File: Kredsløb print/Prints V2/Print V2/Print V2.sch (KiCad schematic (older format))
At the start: 77 parts, among them J1 Conn_01x01_Male, J10 Conn_01x01_Male, J11 Conn_01x01_Male, J12 Conn_01x01_Male, J13 Conn_01x01_Male, J14 Conn_01x01_Male, J15 Conn_01x01_Male, J16 Conn_01x01_Male, J17 Conn_01x01_Male, J18 Conn_01x01_Male, J19 Conn_01x01_Male, J2 Conn_01x01_Male, J20 Conn_01x01_Male, J21 Conn_01x01_Male, J22 Conn_01x01_Male, J23 Conn_01x01_Male, J24 Conn_01x01_Male, J25 Conn_01x01_Male, J26 Conn_01x01_Male, J27 Conn_01x01_Male, J28 Conn_01x01_Male, J29 Conn_01x01_Male, J3 Conn_01x01_Male, J30 Conn_01x01_Male, J31 Conn_01x01_Male, J32 Conn_01x01_Male, J4 Conn_01x01_Male, J5 Conn_01x01_Male, J6 Conn_01x01_Male, J7 Conn_01x01_Male, J8 Conn_01x01_Male, J9 Conn_01x01_Male, Q1 BC547, Q10 TIP120, Q11 TIP127, Q12 TIP120, Q13 TIP127, Q14 TIP120, Q15 BC547, Q16 BC547, Q17 BC547, Q18 TIP127, Q19 TIP120, Q2 BC547, Q20 BC547, Q21 TIP127, Q22 TIP120, Q23 TIP120, Q24 TIP120, Q25 TIP127, Q26 TIP120, Q27 TIP127, Q28 TIP120, Q3 BC547, Q4 TIP127, Q5 TIP120, Q6 BC547, Q7 TIP127, Q8 TIP120, Q9 TIP120, U1 esp32, U2 LM7805_TO220, U3 4049

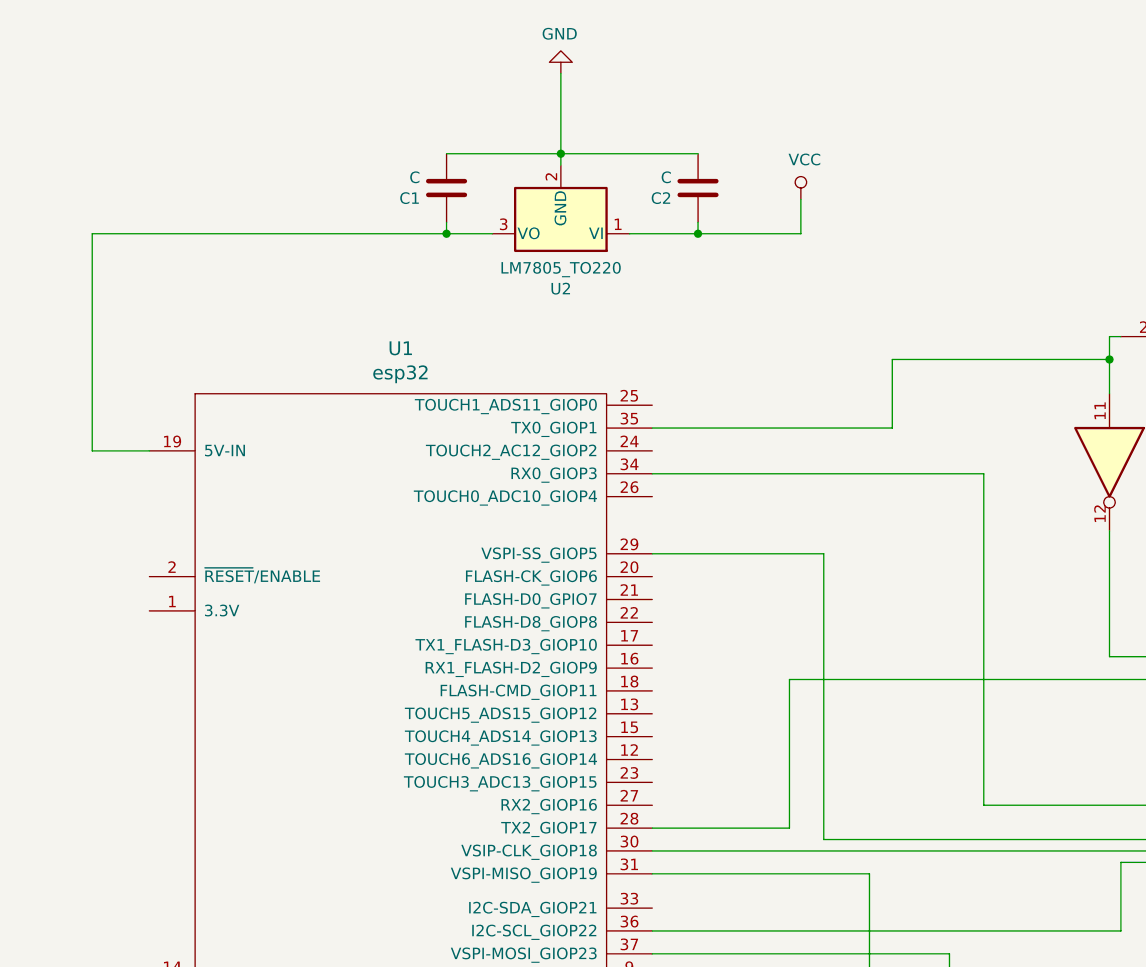
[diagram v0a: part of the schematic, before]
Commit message: kredsløb og ny motor mount
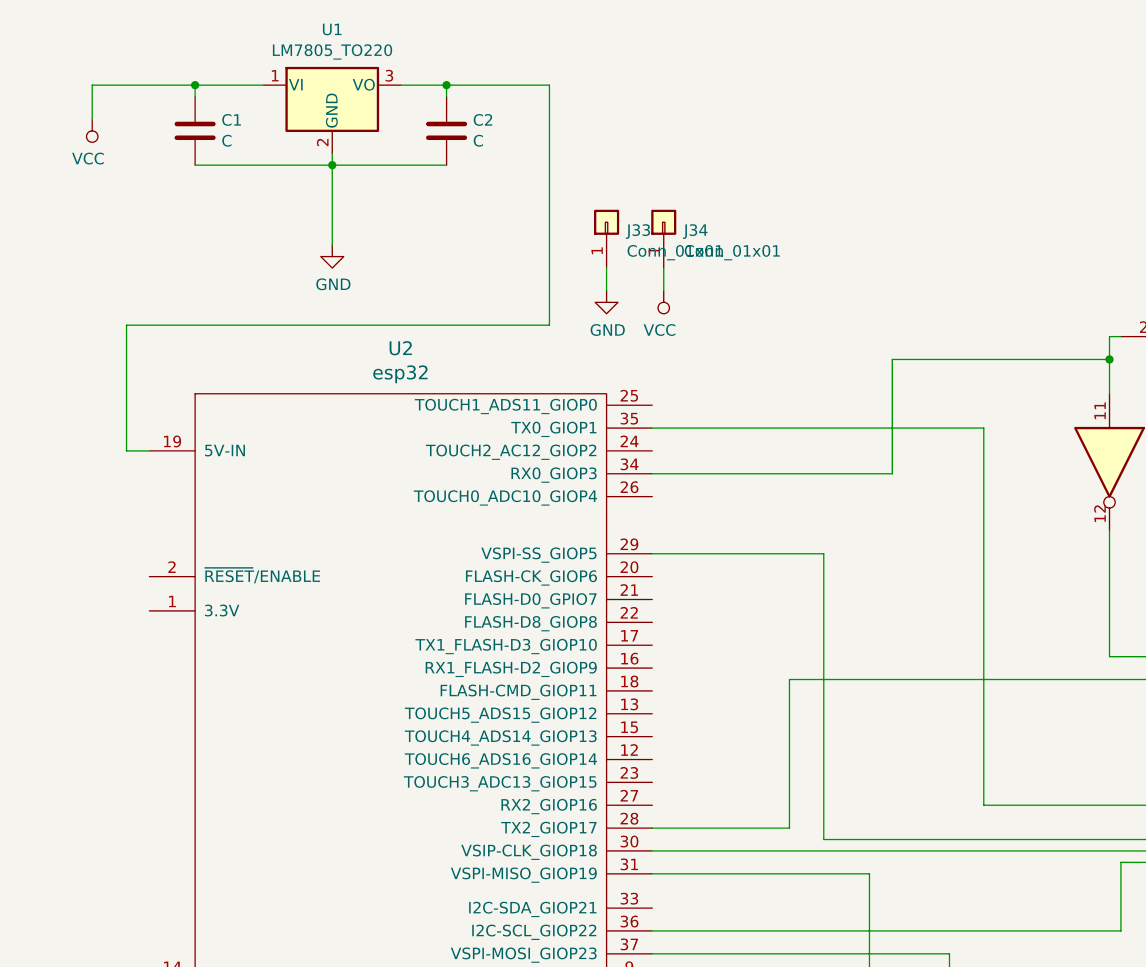
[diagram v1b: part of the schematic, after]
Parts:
- added J33, J34: Conn_01x01, Custom footprints:Power_wire_pad, symbol Connector_Generic:Conn_01x01
- C1: renamed from C2; footprint footprints otg:C_5.00mm -> Custom footprints:C_6.00mm
- C2: renamed from C1; footprint footprints otg:C_5.00mm -> Custom footprints:C_6.00mm
- renumbered U2 to U1, U1 to U2
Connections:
- net GND: now also J33.1 (Pin_1)
- net VCC: now also J34.1 (Pin_1)
- net at Q17.2 (B), U3.9: now also U2.35 (TX0_GIOP1); no longer U2.34 (RX0_GIOP3)
- net at Q3.2 (B), U3.11: now also U2.34 (RX0_GIOP3); no longer U2.35 (TX0_GIOP1)
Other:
- moved on the sheet: C1, C2, U1
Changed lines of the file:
@@
 $EndDescr
 $Comp
-L 00-OTG-Microcontroler:esp32 U1
+L 00-OTG-Microcontroler:esp32 U2
 U 1 1 5C9DC679
 P 2150 3600
-F 0 "U1" H 2150 5347 60  0000 C CNN
+F 0 "U2" H 2150 5347 60  0000 C CNN
 F 1 "esp32" H 2150 5241 60  0000 C CNN
 F 2 "footprints otg:ESP32_mcu" H 2150 3600 60  0001 C CNN
@@
 	5250 1800 5250 1900
 $Comp
-L Regulator_Linear:LM7805_TO220 U2
+L Regulator_Linear:LM7805_TO220 U1
 U 1 1 5CA3A1F0
-P 2850 1350
-F 0 "U2" H 2850 1592 50  0000 C CNN
-F 1 "LM7805_TO220" H 2850 1501 50  0000 C CNN
-F 2 "Package_TO_SOT_THT:TO-220-3_Vertical" H 2850 1575 50  0001 C CIN
-F 3 "http://www.fairchildsemi.com/ds/LM/LM7805.pdf" H 2850 1300 50  0001 C CNN
-	1    2850 1350
-	-1   0    0    1
+P 1850 700
+F 0 "U1" H 1850 942 50  0000 C CNN
+F 1 "LM7805_TO220" H 1850 851 50  0000 C CNN
+F 2 "Package_TO_SOT_THT:TO-220-3_Vertical" H 1850 925 50  0001 C CIN
+F 3 "http://www.fairchildsemi.com/ds/LM/LM7805.pdf" H 1850 650 50  0001 C CNN
+	1    1850 700
+	1    0    0    -1
+$EndComp
+$Comp
+L Device:C C1
+U 1 1 5CA3E782
+P 1250 900
+F 0 "C1" H 1365 946 50  0000 L CNN
+F 1 "C" H 1365 855 50  0000 L CNN
+F 2 "Custom footprints:C_6.00mm" H 1288 750 50  0001 C CNN
+F 3 "~" H 1250 900 50  0001 C CNN
+	1    1250 900
+	1    0    0    -1
 $EndComp
 $Comp
 L Device:C C2
-U 1 1 5CA3E782
-P 3450 1150
-F 0 "C2" H 3565 1196 50  0000 L CNN
-F 1 "C" H 3565 1105 50  0000 L CNN
-F 2 "footprints otg:C_5.00mm" H 3488 1000 50  0001 C CNN
-F 3 "~" H 3450 1150 50  0001 C CNN
-	1    3450 1150
-	-1   0    0    1
-$EndComp
-$Comp
-L Device:C C1
 U 1 1 5CA3FF12
-P 2350 1150
-F 0 "C1" H 2465 1196 50  0000 L CNN
-F 1 "C" H 2465 1105 50  0000 L CNN
-F 2 "footprints otg:C_5.00mm" H 2388 1000 50  0001 C CNN
-F 3 "~" H 2350 1150 50  0001 C CNN
-	1    2350 1150
-	-1   0    0    1
+P 2350 900
+F 0 "C2" H 2465 946 50  0000 L CNN
+F 1 "C" H 2465 855 50  0000 L CNN
+F 2 "Custom footprints:C_6.00mm" H 2388 750 50  0001 C CNN
+F 3 "~" H 2350 900 50  0001 C CNN
+	1    2350 900
+	1    0    0    -1
 $EndComp
 $Comp
 L power:VCC #PWR0102
 U 1 1 5CA41279
-P 3900 1200
-F 0 "#PWR0102" H 3900 1050 50  0001 C CNN
-F 1 "VCC" H 3917 1373 50  0000 C CNN
-F 2 "" H 3900 1200 50  0001 C CNN
-F 3 "" H 3900 1200 50  0001 C CNN
-	1    3900 1200
-	1    0    0    -1
+P 800 850
+F 0 "#PWR0102" H 800 700 50  0001 C CNN
+F 1 "VCC" H 817 1023 50  0000 C CNN
+F 2 "" H 800 850 50  0001 C CNN
+F 3 "" H 800 850 50  0001 C CNN
+	1    800  850
+	-1   0    0    1
 $EndComp
 $Comp
@@
 	6150 4800 6550 4800
 Wire Wire Line
-	3150 1350 3450 1350
-Wire Wire Line
-	3900 1200 3900 1350
-Wire Wire Line
-	3450 1300 3450 1350
-Connection ~ 3450 1350
-Wire Wire Line
-	3450 1350 3900 1350
-Wire Wire Line
-	2350 1300 2350 1350
-Wire Wire Line
-	2350 1350 2550 1350
-Wire Wire Line
-	3450 1000 2850 1000
-Wire Wire Line
-	2850 1050 2850 1000
-Connection ~ 2850 1000
-Wire Wire Line
-	2850 1000 2350 1000
-Wire Wire Line
-	2350 1350 800  1350
-Wire Wire Line
-	800  1350 800  2300
-Wire Wire Line
-	800  2300 1050 2300
-Connection ~ 2350 1350
+	1550 700  1250 700
+Wire Wire Line
+	800  850  800  700
+Wire Wire Line
+	1250 750  1250 700
+Connection ~ 1250 700
+Wire Wire Line
+	1250 700  800  700
+Wire Wire Line
+	2350 750  2350 700
+Wire Wire Line
+	2350 700  2150 700
+Wire Wire Line
+	1250 1050 1850 1050
+Wire Wire Line
+	1850 1000 1850 1050
+Connection ~ 1850 1050
+Wire Wire Line
+	1850 1050 2350 1050
 $Comp
 L 00-OTG-Transistor:BC547 Q15
@@
 $EndComp
 Wire Wire Line
-	3250 2200 4300 2200
-Wire Wire Line
-	4300 2200 4300 1900
-Wire Wire Line
 	4300 1900 5250 1900
 Connection ~ 5250 1900
@@
 	5250 1900 5250 2050
 Wire Wire Line
-	3250 2400 4700 2400
-Wire Wire Line
-	4700 2400 4700 3850
-Wire Wire Line
 	4700 3850 7750 3850
 Wire Wire Line
@@
 Wire Wire Line
 	4200 4150 3250 4150
+Wire Wire Line
+	2350 700  2800 700
+Wire Wire Line
+	2800 700  2800 1750
+Wire Wire Line
+	2800 1750 950  1750
+Wire Wire Line
+	950  1750 950  2300
+Connection ~ 2350 700
+Wire Wire Line
+	950  2300 1050 2300
+Wire Wire Line
+	3250 2400 4300 2400
+Wire Wire Line
+	3250 2200 4700 2200
+Wire Wire Line
+	4300 1900 4300 2400
+Wire Wire Line
+	4700 2200 4700 3850
+Wire Wire Line
+	1850 1400 1850 1050
 $Comp
 L power:GND #PWR0111
 U 1 1 5CD33953
-P 2850 650
-F 0 "#PWR0111" H 2850 400 50  0001 C CNN
-F 1 "GND" H 2855 477 50  0000 C CNN
-F 2 "" H 2850 650 50  0001 C CNN
-F 3 "" H 2850 650 50  0001 C CNN
-	1    2850 650
+P 1850 1400
+F 0 "#PWR0111" H 1850 1150 50  0001 C CNN
+F 1 "GND" H 1855 1227 50  0000 C CNN
+F 2 "" H 1850 1400 50  0001 C CNN
+F 3 "" H 1850 1400 50  0001 C CNN
+	1    1850 1400
+	1    0    0    -1
+$EndComp
+$Comp
+L power:GND #PWR0112
+U 1 1 5CBA879B
+P 3050 1600
+F 0 "#PWR0112" H 3050 1350 50  0001 C CNN
+F 1 "GND" H 3055 1427 50  0000 C CNN
+F 2 "" H 3050 1600 50  0001 C CNN
+F 3 "" H 3050 1600 50  0001 C CNN
+	1    3050 1600
+	1    0    0    -1
+$EndComp
+$Comp
+L power:VCC #PWR0113
+U 1 1 5CBB36DA
+P 3300 1600
+F 0 "#PWR0113" H 3300 1450 50  0001 C CNN
+F 1 "VCC" H 3317 1773 50  0000 C CNN
+F 2 "" H 3300 1600 50  0001 C CNN
+F 3 "" H 3300 1600 50  0001 C CNN
+	1    3300 1600
 	-1   0    0    1
 $EndComp
-Wire Wire Line
-	2850 650  2850 1000
+$Comp
+L Connector_Generic:Conn_01x01 J33
+U 1 1 5CBC9865
+P 3050 1300
+F 0 "J33" V 3014 1212 50  0000 R CNN
+F 1 "Conn_01x01" V 2923 1212 50  0000 R CNN
+F 2 "Custom footprints:Power_wire_pad" H 3050 1300 50  0001 C CNN
+F 3 "~" H 3050 1300 50  0001 C CNN
+	1    3050 1300
+	0    -1   -1   0
+$EndComp
+$Comp
+L Connector_Generic:Conn_01x01 J34
+U 1 1 5CBCB57E
+P 3300 1300
+F 0 "J34" V 3264 1212 50  0000 R CNN
+F 1 "Conn_01x01" V 3173 1212 50  0000 R CNN
+F 2 "Custom footprints:Power_wire_pad" H 3300 1300 50  0001 C CNN
+F 3 "~" H 3300 1300 50  0001 C CNN
+	1    3300 1300
+	0    -1   -1   0
+$EndComp
+Wire Wire Line
+	3050 1600 3050 1500
+Wire Wire Line
+	3300 1600 3300 1500
 $EndSCHEMATC
